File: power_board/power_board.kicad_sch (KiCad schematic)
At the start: 4 parts

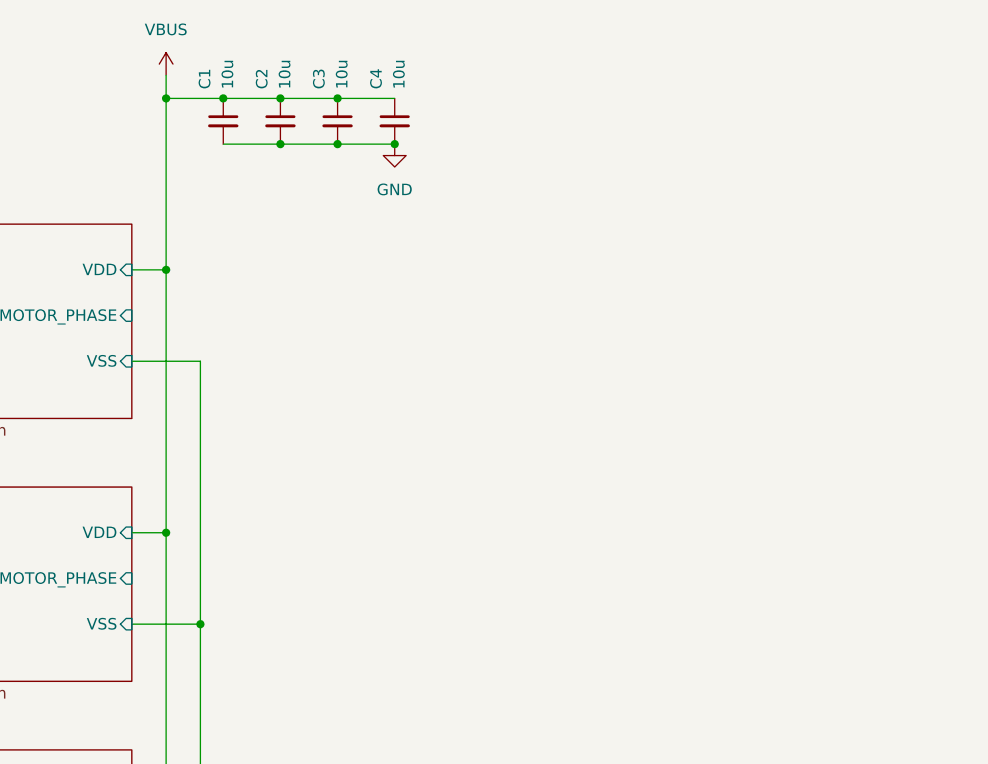
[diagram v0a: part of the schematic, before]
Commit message: Complete primary layout step
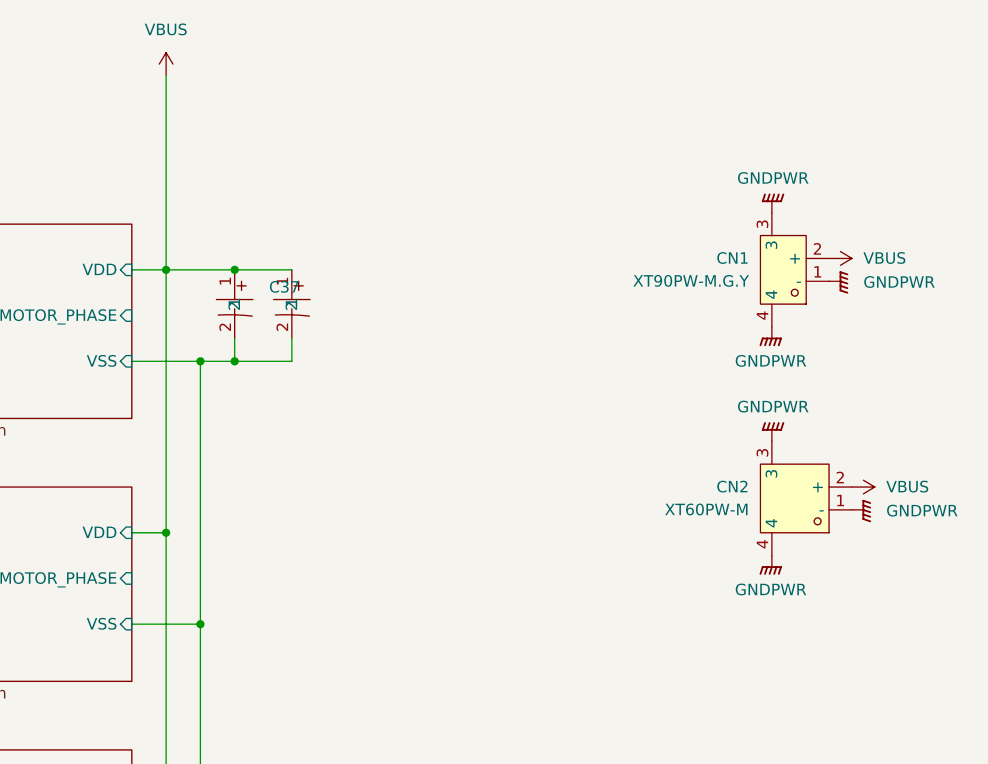
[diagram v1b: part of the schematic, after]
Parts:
- removed C1, C2, C3, C4: 10u, Capacitor_SMD:C_2220_5750Metric, symbol Device:C_Small
- added C37, C38: ERS1KM101G16OT, esc-library:CAP-TH_BD10.0-P5.00-D1.0-FD, symbol esc-library:ERS1KM101G16OT
- added CN1: XT90PW-M.G.Y, esc-library:CONN-TH_XT90PW-M.G.Y, symbol esc-library:XT90PW-M.G.Y
- added CN2: XT60PW-M, esc-library:CONN-TH_XT60PW-M, symbol esc-library:XT60PW-M
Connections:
- net GNDPWR: now also CN1.1 (-), CN1.3, CN1.4, CN2.1 (-), CN2.3, CN2.4
- net VBUS: now also C37.1, C38.1, CN1.2 (+), CN2.2 (+)
- net curret_sense/current+: now also C37.2, C38.2
